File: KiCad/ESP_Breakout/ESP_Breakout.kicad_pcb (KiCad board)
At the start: 2 copper layers, 127 x 70.2 mm, 21 parts, among them J1 Conn_01x15_Socket, J2 Conn_01x15_Socket, J3 Conn_01x03_Pin, J4 Conn_01x03_Pin, J5 Conn_01x03_Pin, J6 Conn_01x03_Pin, J7 Conn_01x15_Socket, J8 Conn_01x15_Socket

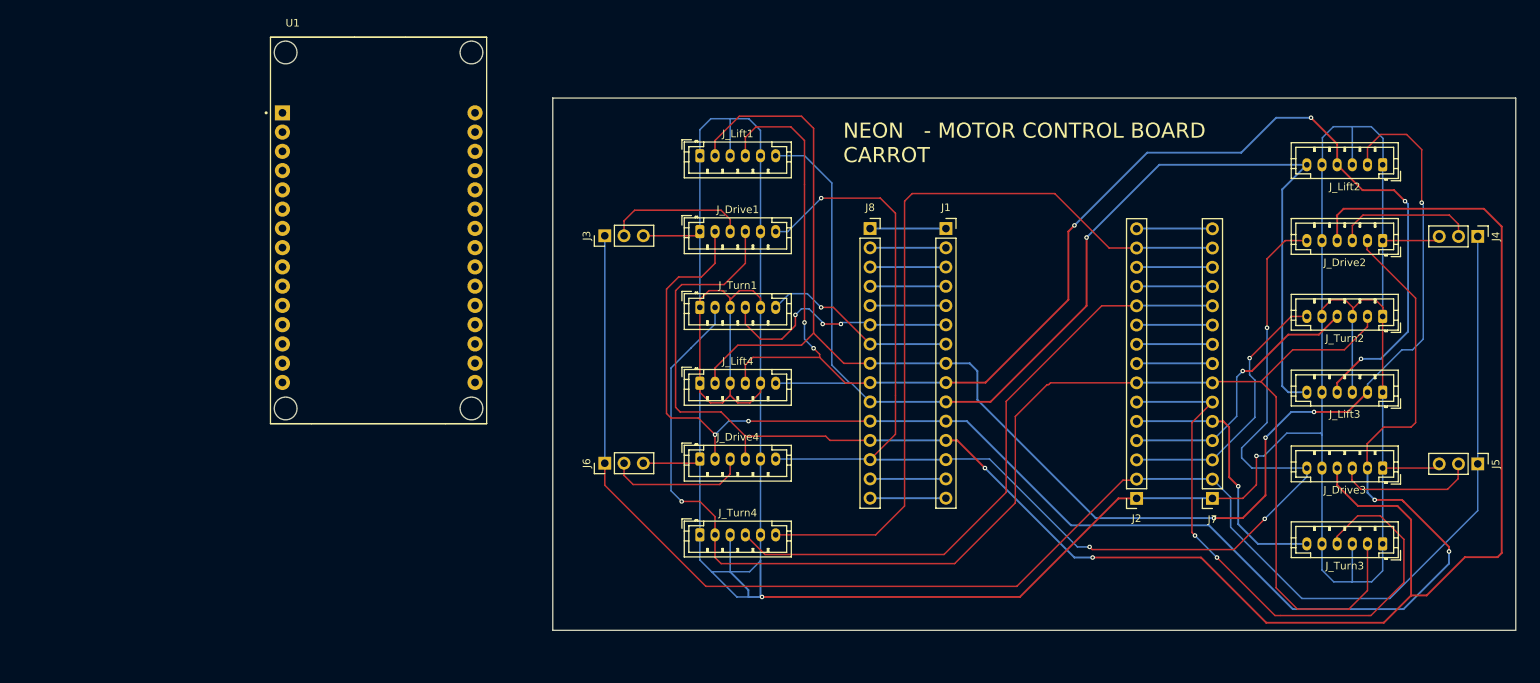
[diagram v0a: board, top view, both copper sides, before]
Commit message: start of pheonix
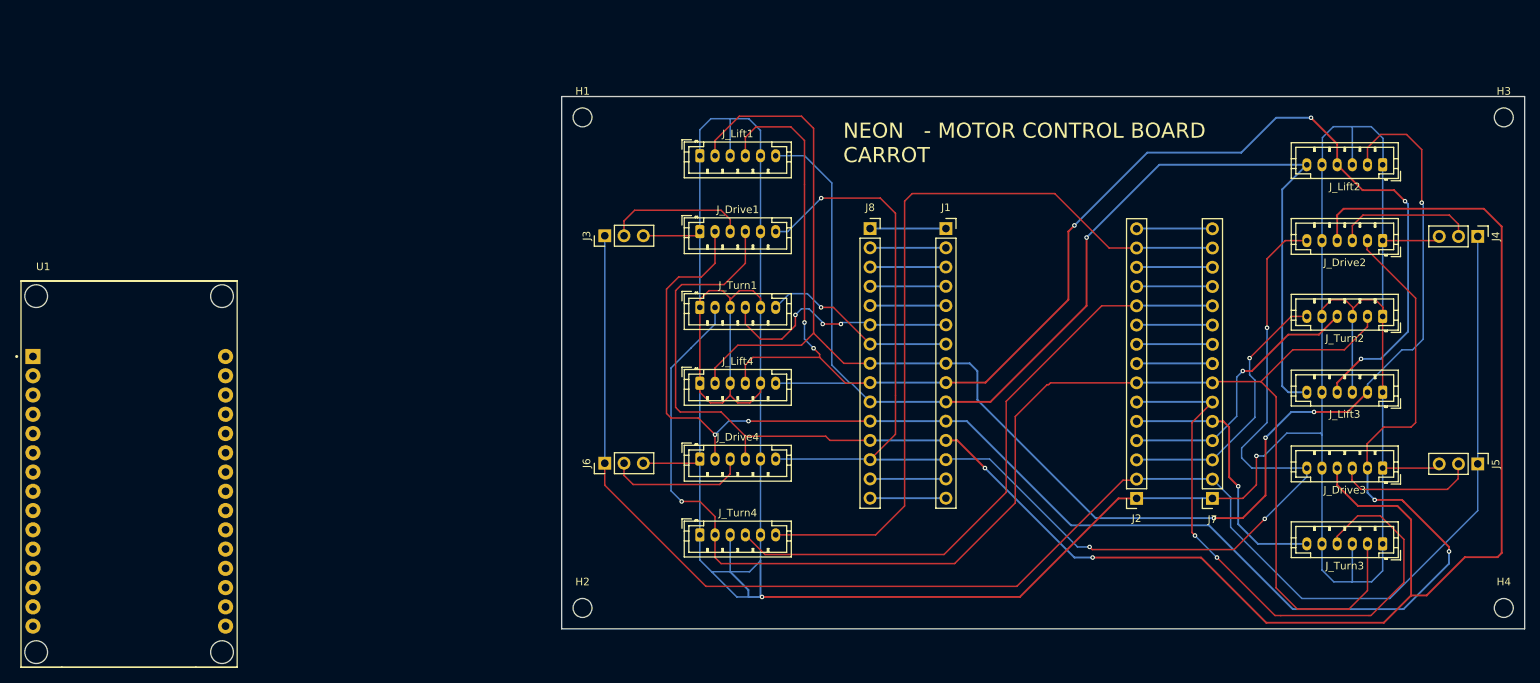
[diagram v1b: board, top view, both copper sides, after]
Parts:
- added H1: MountingHole, MountingHole:MountingHole_2.5mm, F.Cu at (95.9, 48.8)
- added H2: MountingHole, MountingHole:MountingHole_2.5mm, F.Cu at (95.9, 113.5)
- added H3: MountingHole, MountingHole:MountingHole_2.5mm, F.Cu at (217.4, 48.8)
- added H4: MountingHole, MountingHole:MountingHole_2.5mm, F.Cu at (217.4, 113.5)
- moved U1 46.0 mm to (36.1, 95.8)
